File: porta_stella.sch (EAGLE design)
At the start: 105 parts, among them CN4 MicroUSB, IC1 74LS00D, J1 PJ-393, T1 2N3904, T2 PN3906, T3 PN3906, T4 PN3906, T5 MMUN2133LT1G, U1 TPS61090RSAR, U2 MCP73871, X1 SSW-112-02-G-Q

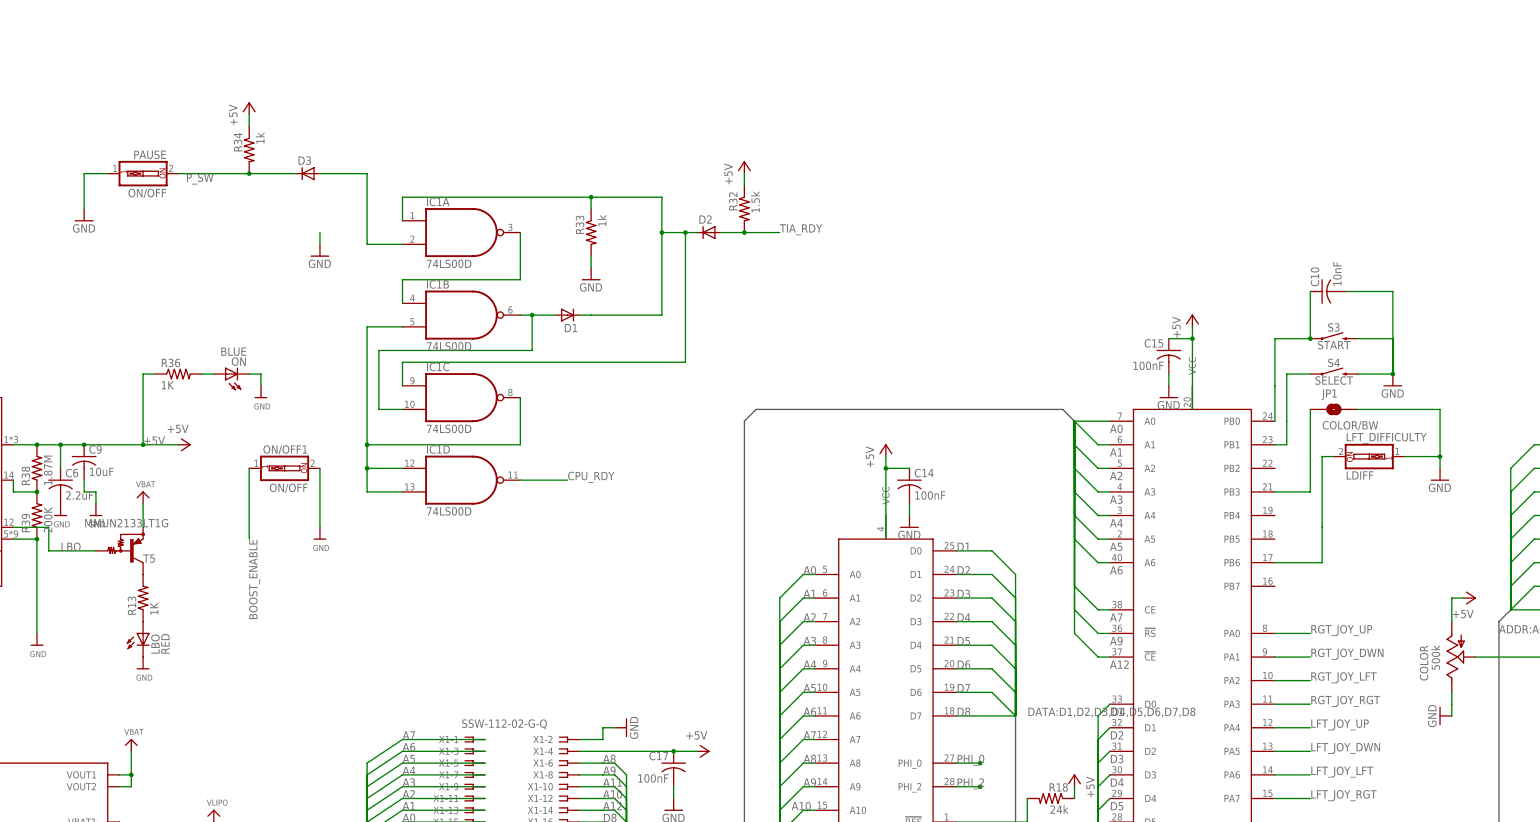
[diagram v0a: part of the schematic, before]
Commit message: Added new switch
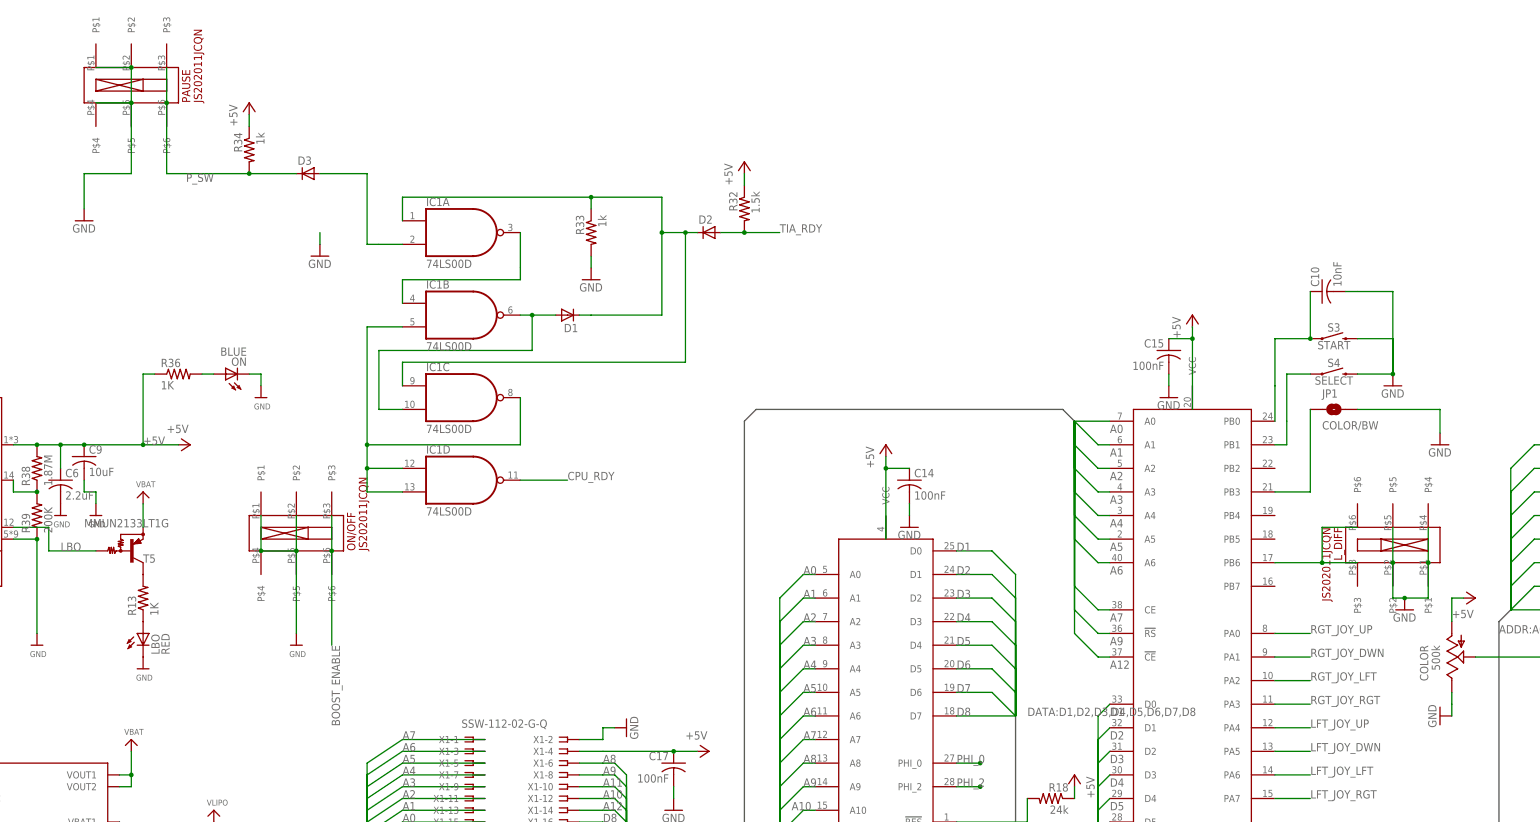
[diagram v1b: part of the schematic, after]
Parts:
- removed LDIFF: LFT_DIFFICULTY, special:SW_DIP-1
- removed ON/OFF1: ON/OFF, special:SW_DIP-1
- added L_DIFF, ON/OFF: JS202011JCQN, tiny_stella:JS202011JCQN
- PAUSE: value ON/OFF -> JS202011JCQN; device special:SW_DIP-1 -> tiny_stella:JS202011JCQN
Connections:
- net BOOST_ENABLE: now also ON/OFF.P$3, ON/OFF.P$6; no longer ON/OFF1.1
- net GND: now also L_DIFF.P$1, L_DIFF.P$2, L_DIFF.P$4, L_DIFF.P$5, ON/OFF.P$1, ON/OFF.P$2, ON/OFF.P$4, ON/OFF.P$5, PAUSE.P$1, PAUSE.P$2, PAUSE.P$4, PAUSE.P$5; no longer LDIFF.1, ON/OFF1.2, PAUSE.1
- net N$21: now also L_DIFF.P$3, L_DIFF.P$6; no longer LDIFF.2
- net P_SW: now also PAUSE.P$3, PAUSE.P$6; no longer PAUSE.2
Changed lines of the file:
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@@
 <part name="GND16" library="supply1" library_urn="urn:adsk.eagle:library:371" deviceset="GND" device=""/>
 <part name="JP1" library="SparkFun-Jumpers" library_urn="urn:adsk.eagle:library:528" deviceset="JUMPER-SMT_2_NO" device="_NO-SILK" package3d_urn="urn:adsk.eagle:package:39277/1" value="COLOR/BW"/>
-<part name="LDIFF" library="special" library_urn="urn:adsk.eagle:library:367" deviceset="SW_DIP-1" device="" package3d_urn="urn:adsk.eagle:package:26661/1" value="LFT_DIFFICULTY"/>
 <part name="GND17" library="supply1" library_urn="urn:adsk.eagle:library:371" deviceset="GND" device=""/>
 <part name="R18" library="resistor" library_urn="urn:adsk.eagle:library:348" deviceset="R-US_" device="M0805" package3d_urn="urn:adsk.eagle:package:26079/1" value="24k"/>
@@
 <part name="R33" library="resistor" library_urn="urn:adsk.eagle:library:348" deviceset="R-US_" device="M0805" package3d_urn="urn:adsk.eagle:package:26079/1" value="1k"/>
 <part name="R34" library="resistor" library_urn="urn:adsk.eagle:library:348" deviceset="R-US_" device="M0805" package3d_urn="urn:adsk.eagle:package:26079/1" value="1k"/>
-<part name="PAUSE" library="special" library_urn="urn:adsk.eagle:library:367" deviceset="SW_DIP-1" device="" package3d_urn="urn:adsk.eagle:package:26661/1" value="ON/OFF"/>
 <part name="D3" library="eagle-ltspice" library_urn="urn:adsk.eagle:library:217" deviceset="DIODE_E-" device="" package3d_urn="urn:adsk.eagle:package:13312/1"/>
 <part name="P+13" library="supply1" library_urn="urn:adsk.eagle:library:371" deviceset="+5V" device=""/>
@@
 <part name="U$25" library="microbuilder" deviceset="GND" device=""/>
 <part name="GND45" library="supply1" deviceset="GND" device=""/>
-<part name="ON/OFF1" library="special" library_urn="urn:adsk.eagle:library:367" deviceset="SW_DIP-1" device="" package3d_urn="urn:adsk.eagle:package:26661/1" value="ON/OFF"/>
 <part name="J1" library="Seeed-Connector" library_urn="urn:adsk.eagle:library:478" deviceset="AUDIO-JACK-PJ-393(8P-SMD)" device="" package3d_urn="urn:adsk.eagle:package:33126/1" value="PJ-393"/>
 <part name="U$5" library="tiny_stella" deviceset="JS5208" device=""/>
+<part name="PAUSE" library="tiny_stella" deviceset="JS202011JCQN" device=""/>
+<part name="ON/OFF" library="tiny_stella" deviceset="JS202011JCQN" device=""/>
+<part name="L_DIFF" library="tiny_stella" deviceset="JS202011JCQN" device=""/>
+<part name="GND2" library="supply1" library_urn="urn:adsk.eagle:library:371" deviceset="GND" device=""/>
 </parts>
 <sheets>
@@
 <instance part="GND16" gate="1" x="83.82" y="91.44"/>
 <instance part="JP1" gate="G$1" x="71.12" y="86.36"/>
-<instance part="LDIFF" gate="G$1" x="78.74" y="76.2" rot="MR180"/>
-<instance part="GND17" gate="1" x="93.98" y="71.12"/>
+<instance part="GND17" gate="1" x="93.98" y="78.74"/>
 <instance part="R18" gate="G$1" x="10.16" y="2.54" rot="MR0"/>
 <instance part="P+14" gate="1" x="15.24" y="7.62" rot="MR0"/>
@@
 <instance part="R33" gate="G$1" x="-88.9" y="124.46" rot="MR270"/>
 <instance part="R34" gate="G$1" x="-162.56" y="142.24" rot="MR270"/>
-<instance part="PAUSE" gate="G$1" x="-185.42" y="137.16" rot="MR0"/>
 <instance part="D3" gate="G$1" x="-149.86" y="137.16" rot="R270"/>
 <instance part="P+13" gate="1" x="-55.88" y="139.7"/>
@@
 <instance part="U2" gate="G$1" x="-208.28" y="-10.16"/>
 <instance part="C22" gate="G$1" x="-246.38" y="-66.04"/>
-<instance part="U$25" gate="G$1" x="-147.32" y="58.42"/>
+<instance part="U$25" gate="G$1" x="-152.4" y="35.56"/>
 <instance part="GND45" gate="1" x="-152.4" y="-50.8"/>
-<instance part="ON/OFF1" gate="G$1" x="-154.94" y="73.66" rot="MR0"/>
 <instance part="J1" gate="G$1" x="312.42" y="17.78"/>
 <instance part="U$5" gate="G$1" x="266.7" y="106.68"/>
+<instance part="PAUSE" gate="G$1" x="-187.96" y="154.94"/>
+<instance part="ON/OFF" gate="G$1" x="-152.4" y="58.42"/>
+<instance part="L_DIFF" gate="G$1" x="83.82" y="58.42" rot="R180"/>
+<instance part="GND2" gate="1" x="86.36" y="43.18"/>
 </instances>
 <busses>
@@
 <pinref part="JP1" gate="G$1" pin="2"/>
 <wire x1="76.2" y1="86.36" x2="93.98" y2="86.36" width="0.1524" layer="91"/>
-<pinref part="LDIFF" gate="G$1" pin="1"/>
-<wire x1="86.36" y1="76.2" x2="93.98" y2="76.2" width="0.1524" layer="91"/>
-<wire x1="93.98" y1="86.36" x2="93.98" y2="76.2" width="0.1524" layer="91"/>
-<wire x1="93.98" y1="76.2" x2="93.98" y2="73.66" width="0.1524" layer="91"/>
-<junction x="93.98" y="76.2"/>
+<wire x1="93.98" y1="86.36" x2="93.98" y2="81.28" width="0.1524" layer="91"/>
 <pinref part="GND17" gate="1" pin="GND"/>
 </segment>
@@
 </segment>
 <segment>
-<pinref part="PAUSE" gate="G$1" pin="1"/>
 <pinref part="GND35" gate="1" pin="GND"/>
-<wire x1="-193.04" y1="137.16" x2="-198.12" y2="137.16" width="0.1524" layer="91"/>
 <wire x1="-198.12" y1="137.16" x2="-198.12" y2="129.54" width="0.1524" layer="91"/>
+<wire x1="-198.12" y1="137.16" x2="-187.96" y2="137.16" width="0.1524" layer="91"/>
+<pinref part="PAUSE" gate="G$1" pin="P$5"/>
+<wire x1="-187.96" y1="137.16" x2="-187.96" y2="152.4" width="0.1524" layer="91"/>
+<pinref part="PAUSE" gate="G$1" pin="P$2"/>
+<wire x1="-187.96" y1="160.02" x2="-187.96" y2="152.4" width="0.1524" layer="91"/>
+<junction x="-187.96" y="152.4"/>
+<pinref part="PAUSE" gate="G$1" pin="P$4"/>
+<wire x1="-187.96" y1="152.4" x2="-195.58" y2="152.4" width="0.1524" layer="91"/>
+<pinref part="PAUSE" gate="G$1" pin="P$1"/>
+<wire x1="-187.96" y1="160.02" x2="-195.58" y2="160.02" width="0.1524" layer="91"/>
+<junction x="-187.96" y="160.02"/>
 </segment>
 <segment>
@@
 <segment>
 <pinref part="U$25" gate="G$1" pin="GND"/>
-<wire x1="-147.32" y1="73.66" x2="-147.32" y2="60.96" width="0.1524" layer="91"/>
-<pinref part="ON/OFF1" gate="G$1" pin="2"/>
+<pinref part="ON/OFF" gate="G$1" pin="P$5"/>
+<wire x1="-152.4" y1="55.88" x2="-152.4" y2="38.1" width="0.1524" layer="91"/>
+<pinref part="ON/OFF" gate="G$1" pin="P$4"/>
+<wire x1="-152.4" y1="55.88" x2="-160.02" y2="55.88" width="0.1524" layer="91"/>
+<junction x="-152.4" y="55.88"/>
+<pinref part="ON/OFF" gate="G$1" pin="P$1"/>
+<wire x1="-160.02" y1="63.5" x2="-160.02" y2="55.88" width="0.1524" layer="91"/>
+<junction x="-160.02" y="55.88"/>
+<pinref part="ON/OFF" gate="G$1" pin="P$2"/>
+<wire x1="-152.4" y1="63.5" x2="-152.4" y2="55.88" width="0.1524" layer="91"/>
 </segment>
 <segment>
 <wire x1="-152.4" y1="-33.02" x2="-152.4" y2="-48.26" width="0.1524" layer="91"/>
 <pinref part="GND45" gate="1" pin="GND"/>
+</segment>
+<segment>
+<pinref part="GND2" gate="1" pin="GND"/>
+<pinref part="L_DIFF" gate="G$1" pin="P$2"/>
+<wire x1="86.36" y1="45.72" x2="83.82" y2="45.72" width="0.1524" layer="91"/>
+<wire x1="83.82" y1="45.72" x2="83.82" y2="53.34" width="0.1524" layer="91"/>
+<wire x1="86.36" y1="45.72" x2="91.44" y2="45.72" width="0.1524" layer="91"/>
+<junction x="86.36" y="45.72"/>
+<pinref part="L_DIFF" gate="G$1" pin="P$1"/>
+<wire x1="91.44" y1="45.72" x2="91.44" y2="53.34" width="0.1524" layer="91"/>
+<pinref part="L_DIFF" gate="G$1" pin="P$4"/>
+<wire x1="91.44" y1="60.96" x2="91.44" y2="53.34" width="0.1524" layer="91"/>
+<junction x="91.44" y="53.34"/>
+<pinref part="L_DIFF" gate="G$1" pin="P$5"/>
+<wire x1="83.82" y1="60.96" x2="83.82" y2="53.34" width="0.1524" layer="91"/>
+<junction x="83.82" y="53.34"/>
 </segment>
 </net>
@@
 <wire x1="58.42" y1="53.34" x2="68.58" y2="53.34" width="0.1524" layer="91"/>
 <wire x1="68.58" y1="53.34" x2="68.58" y2="60.96" width="0.1524" layer="91"/>
-<pinref part="LDIFF" gate="G$1" pin="2"/>
-<wire x1="71.12" y1="76.2" x2="68.58" y2="76.2" width="0.1524" layer="91"/>
-<wire x1="68.58" y1="76.2" x2="68.58" y2="60.96" width="0.1524" layer="91"/>
+<pinref part="L_DIFF" gate="G$1" pin="P$6"/>
+<wire x1="76.2" y1="60.96" x2="68.58" y2="60.96" width="0.1524" layer="91"/>
+<pinref part="L_DIFF" gate="G$1" pin="P$3"/>
+<wire x1="76.2" y1="53.34" x2="68.58" y2="53.34" width="0.1524" layer="91"/>
+<junction x="68.58" y="53.34"/>
 </segment>
 </net>
@@
 <segment>
 <pinref part="R34" gate="G$1" pin="2"/>
-<pinref part="PAUSE" gate="G$1" pin="2"/>
-<wire x1="-162.56" y1="137.16" x2="-177.8" y2="137.16" width="0.1524" layer="91"/>
+<wire x1="-162.56" y1="137.16" x2="-180.34" y2="137.16" width="0.1524" layer="91"/>
 <label x="-170.18" y="137.16" size="1.778" layer="95" rot="R180"/>
 <pinref part="D3" gate="G$1" pin="A"/>
 <wire x1="-152.4" y1="137.16" x2="-162.56" y2="137.16" width="0.1524" layer="91"/>
 <junction x="-162.56" y="137.16"/>
+<pinref part="PAUSE" gate="G$1" pin="P$6"/>
+<wire x1="-180.34" y1="137.16" x2="-180.34" y2="152.4" width="0.1524" layer="91"/>
+<pinref part="PAUSE" gate="G$1" pin="P$3"/>
+<wire x1="-180.34" y1="152.4" x2="-180.34" y2="160.02" width="0.1524" layer="91"/>
+<junction x="-180.34" y="152.4"/>
 </segment>
 <segment>
@@
 </segment>
 <segment>
-<label x="-162.56" y="58.42" size="1.778" layer="95" rot="R270"/>
-<wire x1="-162.56" y1="58.42" x2="-162.56" y2="73.66" width="0.1524" layer="91"/>
-<pinref part="ON/OFF1" gate="G$1" pin="1"/>
-</segment>
-</net>
+<label x="-144.78" y="35.56" size="1.778" layer="95" rot="R270"/>
+<pinref part="ON/OFF" gate="G$1" pin="P$6"/>
+<wire x1="-144.78" y1="55.88" x2="-144.78" y2="35.56" width="0.1524" layer="91"/>
+<pinref part="ON/OFF" gate="G$1" pin="P$3"/>
+<wire x1="-144.78" y1="55.88" x2="-144.78" y2="63.5" width="0.1524" layer="91"/>
+<junction x="-144.78" y="55.88"/>
+</segment>
+</net>

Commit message: ready to finish wiring
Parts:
- removed GND_V: GND_V, wirepad:WIREPAD2,54/1,1
- removed S2: L_FIRE, SparkFun-Switches:MOMENTARY-SWITCH-SPST-SMD-5.2MM
- added GND_CVID: GND_CVID, wirepad:WIREPAD2,54/1,1
- added J2: SJ-43516-SMT, tiny_stella:SJ-43516-SMT
- added SW1: E-SWITCH_JS5208E-SWITCH_JS5208_0_0, tiny_stella:E-SWITCH_JS5208E-SWITCH_JS5208_0_0
- added U$7: TL3300DF260Q, tiny_stella:TL3300DF260Q
- J1: value PJ-393 -> 2p-smd-1.0-90d; device Seeed-Connector:AUDIO-JACK-PJ-393(8P-SMD) -> Seeed-Connector:SMD-JST-2P-1.0-90D
- U$5: value JS5208 -> 3352P-1-103LF; device tiny_stella:JS5208 -> tiny_stella:3352P-1-103LF
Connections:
- net N$8 renamed RAW_CVID
- new net AUD: J2.RING1, J2.TIP, U$5.A
- new net CVID: J2.SLEEVE
- new net JACK_AUD_OUT_L: J2.TIP_SWITCH
- new net JACK_AUD_OUT_R: J2.RING_SWITCH
- new net N$56: SW1.4
- new net N$8: AUD.P
- net GND: now also GND_CVID.P, J1.2, J2.RING2, SW1.PUSH(N.O.), U$5.E, U$7.P$3, U$7.P$4; no longer GND_V.P, S2.2, U$5.GND
- net LFT_FIRE: now also U$7.P$1, U$7.P$2; no longer S2.1
- net LFT_JOY_DWN: now also SW1.2; no longer U$5.C-D
- net LFT_JOY_LFT: now also SW1.6; no longer U$5.B-L
- net LFT_JOY_RGT: now also SW1.5; no longer U$5.D-R
- net LFT_JOY_UP: now also SW1.COMM.; no longer U$5.A-U
- net N$28: now also U$5.S; no longer AUD.P
- net VLIPO: now also J1.1
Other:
- note added: "Atari 2600"
- note added: "Battery and Power Circuitry Referenced from the Powerboost 1000 By Adafruit"
- note added: "Composite Video Amplifier By Simon Plata"
- note added: "Pause Switch Circuitry By Victor Trucco www.victortrucco.com"
- moved on the sheet: AUD, BRIGHT, C1, C10, C11, C14, C15, C16, C17, C18, C19, C2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
